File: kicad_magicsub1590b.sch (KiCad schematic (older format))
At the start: 18 parts, among them P1 EXT_IO, P2 EXT_IO, P3 M3Drill, P4 M3Drill, P5 EXT_IO, P6 M3Drill, P7 M3Drill, P8 EXT_IO, U1 B10k, U2 B10k, U3 B10k

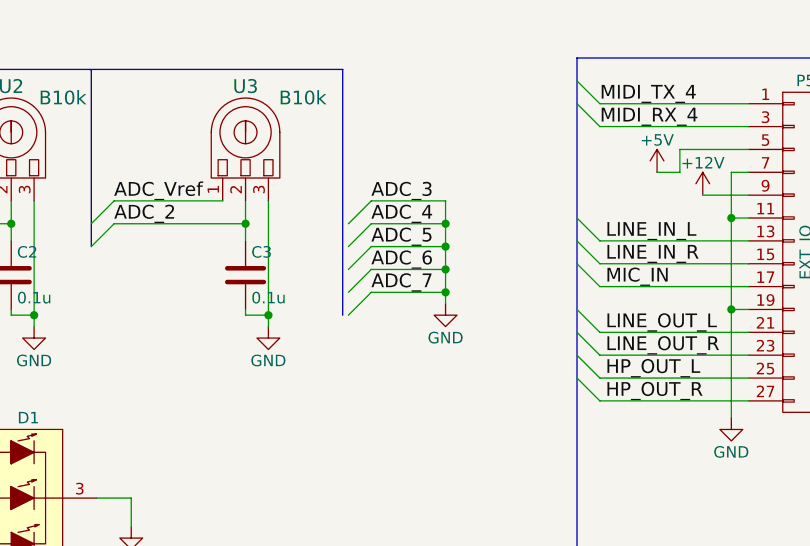
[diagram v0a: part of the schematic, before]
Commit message: 配線引いた
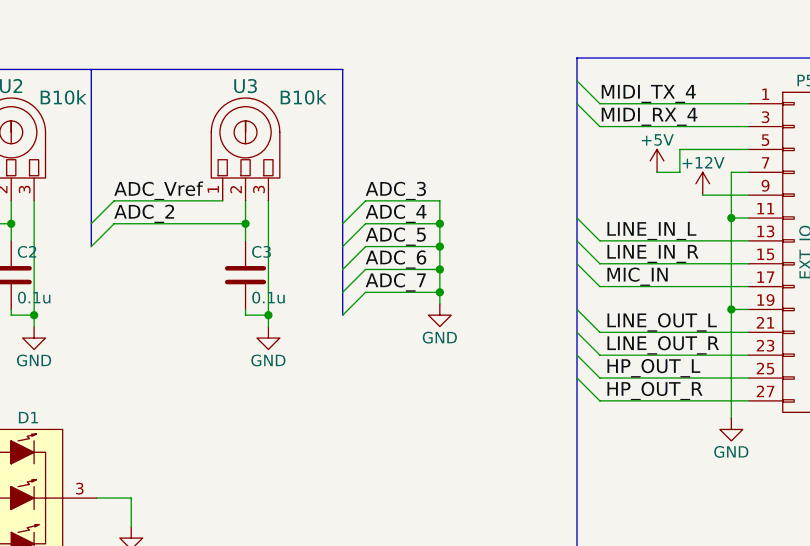
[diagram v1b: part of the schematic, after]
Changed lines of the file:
@@
 LIBS:hastech
 LIBS:kamiya
-LIBS:kicad_magicsub1690b-cache
+LIBS:kicad_magicsub1590b-cache
 EELAYER 25 0
 EELAYER END
@@
 Wire Wire Line
 	5450 3275 5875 3275
-Text Label 8100 1775 0    60   ~ 0
+Text Label 8075 1775 0    60   ~ 0
 ADC_3
-Text Label 8100 1875 0    60   ~ 0
+Text Label 8075 1875 0    60   ~ 0
 ADC_4
-Text Label 8100 1975 0    60   ~ 0
+Text Label 8075 1975 0    60   ~ 0
 ADC_5
-Text Label 8100 2075 0    60   ~ 0
+Text Label 8075 2075 0    60   ~ 0
 ADC_6
-Text Label 8100 2175 0    60   ~ 0
+Text Label 8075 2175 0    60   ~ 0
 ADC_7
 $Comp
 L GND #PWR12
 U 1 1 586156CC
-P 8425 2225
-F 0 "#PWR12" H 8425 1975 50  0001 C CNN
-F 1 "GND" H 8425 2075 50  0000 C CNN
-F 2 "" H 8425 2225 50  0000 C CNN
-F 3 "" H 8425 2225 50  0000 C CNN
-	1    8425 2225
-	1    0    0    -1
-$EndComp
-Wire Wire Line
-	8100 1775 8425 1775
-Wire Wire Line
-	8425 1775 8425 2225
-Wire Wire Line
-	8100 1875 8425 1875
-Connection ~ 8425 1875
-Connection ~ 8425 1975
-Connection ~ 8425 2075
-Connection ~ 8425 2175
-Wire Wire Line
-	8100 1975 8425 1975
-Wire Wire Line
-	8100 2075 8425 2075
-Wire Wire Line
-	8100 2175 8425 2175
+P 8400 2225
+F 0 "#PWR12" H 8400 1975 50  0001 C CNN
+F 1 "GND" H 8400 2075 50  0000 C CNN
+F 2 "" H 8400 2225 50  0000 C CNN
+F 3 "" H 8400 2225 50  0000 C CNN
+	1    8400 2225
+	1    0    0    -1
+$EndComp
+Wire Wire Line
+	8075 1775 8400 1775
+Wire Wire Line
+	8400 1775 8400 2225
+Wire Wire Line
+	8075 1875 8400 1875
+Connection ~ 8400 1875
+Connection ~ 8400 1975
+Connection ~ 8400 2075
+Connection ~ 8400 2175
+Wire Wire Line
+	8075 1975 8400 1975
+Wire Wire Line
+	8075 2075 8400 2075
+Wire Wire Line
+	8075 2175 8400 2175
 $Comp
 L CONN_02X14 P2
@@
 	6875 1975 6975 1875
 Entry Wire Line
-	8000 1875 8100 1775
-Entry Wire Line
-	8000 1975 8100 1875
-Entry Wire Line
-	8000 2075 8100 1975
-Entry Wire Line
-	8000 2175 8100 2075
-Entry Wire Line
-	8000 2275 8100 2175
+	7975 1875 8075 1775
+Entry Wire Line
+	7975 1975 8075 1875
+Entry Wire Line
+	7975 2075 8075 1975
+Entry Wire Line
+	7975 2175 8075 2075
+Entry Wire Line
+	7975 2275 8075 2175
 Wire Bus Line
 	7975 1200 7975 2275
